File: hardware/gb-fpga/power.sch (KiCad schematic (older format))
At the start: 39 parts, among them J3 BAT+, J4 BAT-, Q1 MBT3904DW1, SW1 SW_SPST, U4 LTC3555, U5 TLV61046ADB

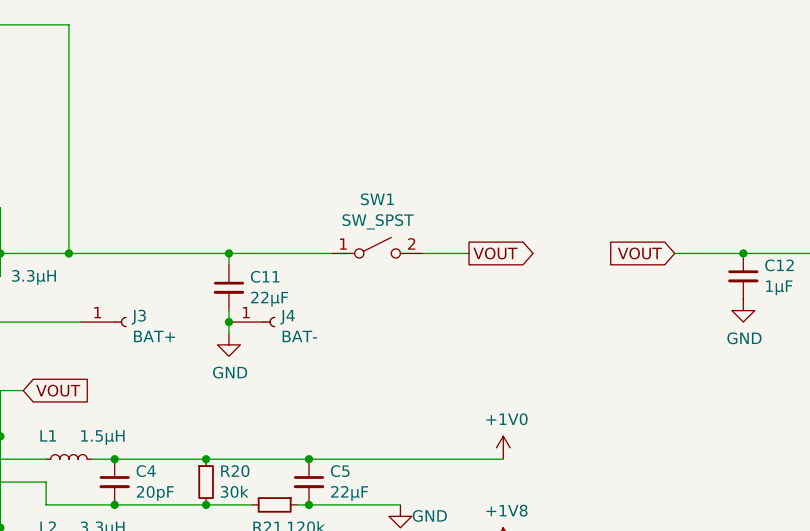
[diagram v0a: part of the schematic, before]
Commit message: Add power switch
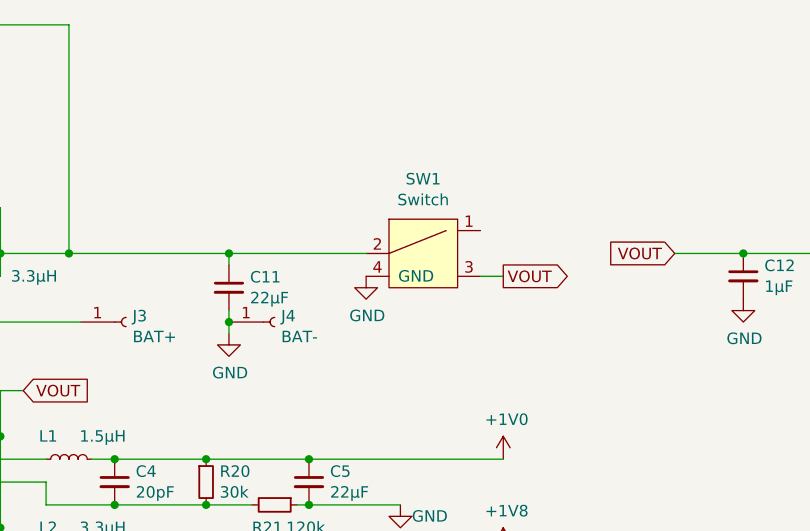
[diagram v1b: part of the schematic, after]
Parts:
- removed SW1: SW_SPST, symbol Switch:SW_SPST
- added SW1: Switch, gb-fpga:EG2215, symbol gb-fpga:Switch
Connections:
- net GND: now also SW1.4 (GND)
- net VOUT: now also SW1.3
- net at C11.1, L4.2, R32.1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: now also SW1.2
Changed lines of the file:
@@
 	1    0    0    -1
 $EndComp
-Text GLabel 7550 2800 2    50   Output ~ 0
+Text GLabel 7700 2900 2    50   Output ~ 0
 VOUT
 Wire Wire Line
-	7550 2800 7350 2800
+	7700 2900 7600 2900
 Text GLabel 1450 3600 0    50   Input ~ 0
 VOUT
@@
 	1    0    0    -1
 $EndComp
-$Comp
-L Switch:SW_SPST SW1
-U 1 1 60E48A72
-P 7150 2800
-F 0 "SW1" H 7150 3035 50  0000 C CNN
-F 1 "SW_SPST" H 7150 2944 50  0000 C CNN
-F 2 "" H 7150 2800 50  0001 C CNN
-F 3 "~" H 7150 2800 50  0001 C CNN
-	1    7150 2800
-	1    0    0    -1
-$EndComp
-Wire Wire Line
-	6950 2800 6500 2800
+Wire Wire Line
+	7100 2800 6500 2800
 Wire Wire Line
 	1600 3600 3800 3600
@@
 	9150 3400 9200 3400
 Connection ~ 9150 3200
+$Comp
+L gb-fpga:Switch SW1
+U 1 1 60DEB027
+P 7350 2800
+F 0 "SW1" H 7350 3125 50  0000 C CNN
+F 1 "Switch" H 7350 3034 50  0000 C CNN
+F 2 "gb-fpga:EG2215" H 7350 2800 50  0001 C CNN
+F 3 "" H 7350 2800 50  0001 C CNN
+	1    7350 2800
+	1    0    0    -1
+$EndComp
+$Comp
+L power:GND #PWR0185
+U 1 1 60E05727
+P 7100 2900
+F 0 "#PWR0185" H 7100 2650 50  0001 C CNN
+F 1 "GND" H 7105 2727 50  0000 C CNN
+F 2 "" H 7100 2900 50  0001 C CNN
+F 3 "" H 7100 2900 50  0001 C CNN
+	1    7100 2900
+	1    0    0    -1
+$EndComp
 $EndSCHEMATC
